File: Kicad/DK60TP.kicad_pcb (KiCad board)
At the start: 2 copper layers, 285 x 113.5 mm, 333 parts, among them J1 USB_mini_micro_B, J2 RGB, J3 CAPS_LOCK, K0 K00, K10 K10, K100 K01, K110 K11, K120 K21, K130 K31, K140 K41, K141 K41, K20 K20, K200 K02, K21 K20, K210 K12, K220 K22, K230 K32, K240 K42, K241 K42, K30 K30, K300 K03, K31 K30, K310 K13, K320 K23, K330 K33, K340 LMB, K341 LMB, K40 K40, K400 K04, K41 K40, K410 K14, K420 K24, K430 K34, K440 MMB, K4C1 K4C, K500 K05, K510 K15, K520 K25, K530 K35, K540 K45, K600 K06, K610 K16, K620 K26, K630 K36, K640 K46, K641 K46, K642 K46, K643 K46, K700 K07, K710 K17, K720 K27, K730 K37, K740 K47, K800 K08, K810 K18, K820 K28, K830 K38, K840 RMB, K841 RMB, K900 K09, K910 K19, K920 K29, K930 K39, K940 K49, M1 MISC, M2 MISC, P1 MOUSE_BOARD, P2 MAIN_BOARD, P3 TRACKPOINT, SW1 RESET, U0 ATMEGA32U4-MU, U1 PAM2804, Y1 Crystal

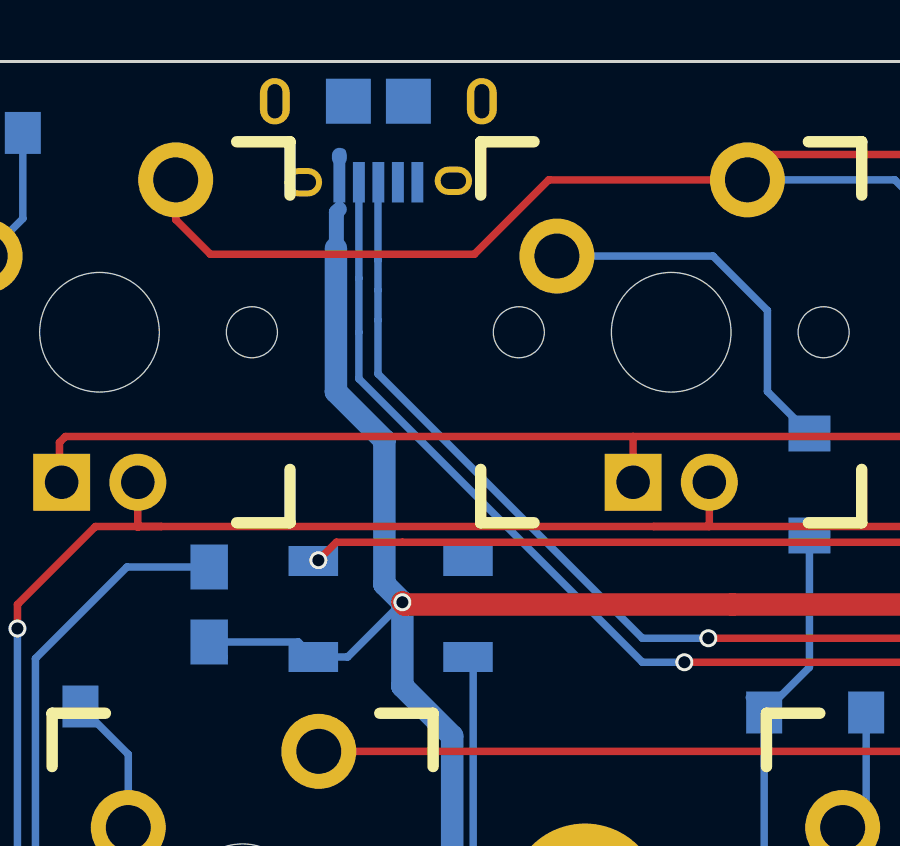
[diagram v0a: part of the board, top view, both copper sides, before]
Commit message: Fixed position of the USB port
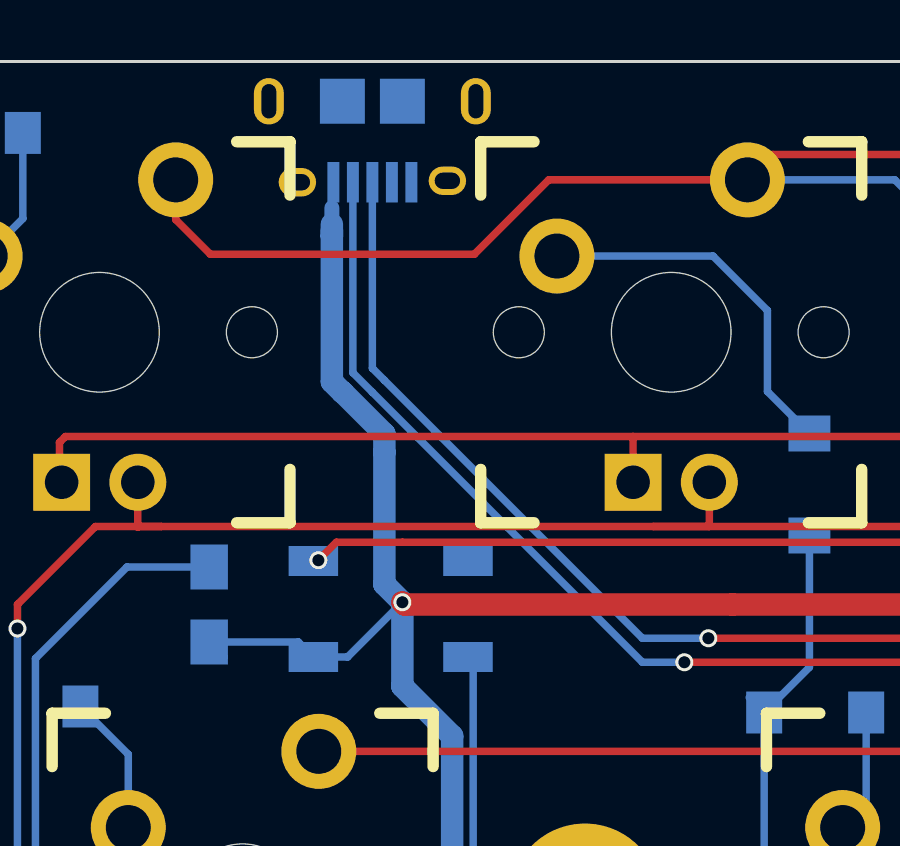
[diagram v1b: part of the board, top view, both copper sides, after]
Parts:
- moved J1 0.20 mm to (82.0, 44.0)
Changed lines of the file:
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@@
     (links 583)
     (no_connects 2)
-    (area 63.881249 39.906249 348.981251 153.506251)
+    (area 44.081251 23.35625 382.58125 192.356251)
     (thickness 1.6)
     (drawings 55)
-    (tracks 2668)
+    (tracks 2666)
     (zones 0)
     (modules 333)
@@
     (38 B.Mask user)
     (39 F.Mask user)
-    (40 Dwgs.User user)
+    (40 Dwgs.User user hide)
     (41 Cmts.User user)
     (42 Eco1.User user)
@@
   )
   (module Footprint:Micro_USB_Hand (layer B.Cu)
-    (at 82.245 43.98125 180)
+    (at 82.045 43.98125 180)
     (fp_text reference J1 (at 0 -2.05 180) (layer B.SilkS)
       (effects (font (size 1 1) (thickness 0.15)) (justify mirror))
@@
   (segment (start 141.931517 126.560413) (end 142.627354 127.25625) (width 0.25) (layer B.Cu) (net 5) (status 10))
   (segment (start 141.909163 126.560413) (end 141.917913 126.560413) (width 0.25) (layer B.Cu) (net 5) (status 30))
+  (segment (start 80.694998 44.831248) (end 80.694998 44.031252) (width 0.25) (layer B.Cu) (net 6) (status 800000))
+  (segment (start 80.694998 44.031252) (end 80.745 43.98125) (width 0.25) (layer B.Cu) (net 6) (status C00000))
+  (segment (start 80.694998 45.38125) (end 80.694998 44.831248) (width 0.5) (layer B.Cu) (net 6))
+  (segment (start 80.694998 45.78125) (end 80.694998 45.38125) (width 0.75) (layer B.Cu) (net 6))
+  (segment (start 81.045 50.98125) (end 81.055048 50.98125) (width 0.75) (layer B.Cu) (net 6))
+  (segment (start 82.445 52.371202) (end 82.445 52.98125) (width 0.75) (layer B.Cu) (net 6))
+  (segment (start 81.055048 50.98125) (end 82.445 52.371202) (width 0.75) (layer B.Cu) (net 6))
+  (segment (start 80.694998 50.631248) (end 80.694998 45.78125) (width 0.75) (layer B.Cu) (net 6))
+  (segment (start 80.694998 45.78125) (end 80.694998 45.58125) (width 0.75) (layer B.Cu) (net 6))
+  (segment (start 81.045 50.98125) (end 80.694998 50.631248) (width 0.75) (layer B.Cu) (net 6))
+  (segment (start 80.745 43.98125) (end 80.745 44.48125) (width 0.25) (layer B.Cu) (net 6) (status C00000))
   (segment (start 80.078 59.80625) (end 81.22 59.80625) (width 0.25) (layer B.Cu) (net 6))
   (segment (start 81.22 59.80625) (end 83.045 57.98125) (width 0.25) (layer B.Cu) (net 6))
@@
   (segment (start 83.12 58.05625) (end 83.045 57.98125) (width 0.75) (layer F.Cu) (net 6))
   (via (at 83.045 57.98125) (size 0.6) (drill 0.4) (layers F.Cu B.Cu) (net 6))
-  (segment (start 82.445 52.58125) (end 80.829375 50.965625) (width 0.75) (layer B.Cu) (net 6))
-  (segment (start 80.845 46.18125) (end 80.829375 46.18125) (width 0.5) (layer B.Cu) (net 6))
-  (segment (start 80.845 44.98125) (end 80.945 44.88125) (width 0.5) (layer B.Cu) (net 6))
-  (segment (start 80.829375 46.18125) (end 80.829375 50.965625) (width 0.75) (layer B.Cu) (net 6))
-  (segment (start 80.945 43.98125) (end 80.945 44.88125) (width 0.25) (layer B.Cu) (net 6))
-  (segment (start 80.845 44.98125) (end 80.845 46.18125) (width 0.5) (layer B.Cu) (net 6))
   (segment (start 83.045 57.98125) (end 82.445 57.38125) (width 0.75) (layer B.Cu) (net 6))
-  (segment (start 82.445 57.38125) (end 82.445 52.58125) (width 0.75) (layer B.Cu) (net 6))
-  (segment (start 80.945 43.18125) (end 80.945 43.08125) (width 0.5) (layer B.Cu) (net 6))
-  (segment (start 80.945 43.98125) (end 80.945 43.18125) (width 0.25) (layer B.Cu) (net 6))
-  (segment (start 80.945 43.08125) (end 81.045 42.98125) (width 0.25) (layer B.Cu) (net 6))
+  (segment (start 82.445 57.38125) (end 82.445 52.98125) (width 0.75) (layer B.Cu) (net 6))
   (segment (start 302.41375 108.85625) (end 302.41375 111.15) (width 0.25) (layer B.Cu) (net 6))
   (segment (start 308.77 117.50625) (end 319.005 117.50625) (width 0.25) (layer B.Cu) (net 6))
@@
   (segment (start 331.705 122.02) (end 331.08375 122.64125) (width 0.25) (layer B.Cu) (net 91) (status 30))
   (segment (start 331.08375 122.64125) (end 333.465 122.64125) (width 0.25) (layer B.Cu) (net 91) (status 30))
+  (segment (start 81.395 43.98125) (end 81.395 50.33125) (width 0.25) (layer B.Cu) (net 92) (status 400000))
+  (segment (start 81.395 50.33125) (end 82.045 50.98125) (width 0.25) (layer B.Cu) (net 92))
   (segment (start 125.445 60.38125) (end 127.81375 62.75) (width 0.25) (layer B.Cu) (net 92))
   (segment (start 127.81375 62.75) (end 127.81375 67.18125) (width 0.25) (layer B.Cu) (net 92))
@@
   (via (at 125.445 60.38125) (size 0.6) (drill 0.4) (layers F.Cu B.Cu) (net 92))
   (segment (start 125.045 59.98125) (end 125.445 60.38125) (width 0.25) (layer F.Cu) (net 92))
-  (segment (start 81.595 48.98125) (end 81.595 50.53125) (width 0.25) (layer B.Cu) (net 92))
-  (segment (start 81.595 50.53125) (end 91.045 59.98125) (width 0.25) (layer B.Cu) (net 92))
+  (segment (start 82.045 50.98125) (end 91.045 59.98125) (width 0.25) (layer B.Cu) (net 92))
   (via (at 92.445 59.98125) (size 0.6) (drill 0.4) (layers F.Cu B.Cu) (net 92))
   (segment (start 91.045 59.98125) (end 92.445 59.98125) (width 0.25) (layer B.Cu) (net 92))
-  (segment (start 81.595 47.18125) (end 81.595 48.98125) (width 0.25) (layer B.Cu) (net 92))
-  (segment (start 81.595 43.98125) (end 81.595 47.18125) (width 0.25) (layer B.Cu) (net 92))
+  (segment (start 82.045 43.98125) (end 82.045 50.18125) (width 0.25) (layer B.Cu) (net 93) (status 400000))
+  (segment (start 82.045 50.18125) (end 82.445 50.58125) (width 0.25) (layer B.Cu) (net 93))
   (segment (start 123.245 59.18125) (end 125.445 59.18125) (width 0.25) (layer F.Cu) (net 93))
   (segment (start 125.445 59.18125) (end 127.045 60.78125) (width 0.25) (layer F.Cu) (net 93))
-  (segment (start 82.23125 48.58125) (end 82.23125 50.3675) (width 0.25) (layer B.Cu) (net 93))
   (segment (start 123.045 59.18125) (end 123.245 59.18125) (width 0.25) (layer F.Cu) (net 93))
   (segment (start 109.445 59.18125) (end 123.045 59.18125) (width 0.25) (layer F.Cu) (net 93))
@@
   (via (at 93.245 59.18125) (size 0.6) (drill 0.4) (layers F.Cu B.Cu) (net 93))
   (segment (start 91.045 59.18125) (end 93.245 59.18125) (width 0.25) (layer B.Cu) (net 93))
-  (segment (start 82.23125 50.3675) (end 91.045 59.18125) (width 0.25) (layer B.Cu) (net 93))
+  (segment (start 82.445 50.58125) (end 91.045 59.18125) (width 0.25) (layer B.Cu) (net 93))
   (segment (start 128.263752 62.000002) (end 128.263752 62.78125) (width 0.25) (layer B.Cu) (net 93))
   (segment (start 127.045 60.78125) (end 128.263752 62.000002) (width 0.25) (layer B.Cu) (net 93))
@@
   (segment (start 128.263752 74.869854) (end 128.263752 62.78125) (width 0.25) (layer B.Cu) (net 93))
   (segment (start 135.109158 81.71526) (end 128.263752 74.869854) (width 0.25) (layer B.Cu) (net 93))
-  (segment (start 82.23125 47.58125) (end 82.23125 48.58125) (width 0.25) (layer B.Cu) (net 93))
-  (segment (start 82.23125 46.58125) (end 82.23125 43.995) (width 0.25) (layer B.Cu) (net 93))
-  (segment (start 82.23125 43.995) (end 82.245 43.98125) (width 0.25) (layer B.Cu) (net 93))
-  (segment (start 82.23125 47.58125) (end 82.23125 46.58125) (width 0.25) (layer B.Cu) (net 93))
   (segment (start 311.445 117.631252) (end 320.194998 117.631252) (width 0.25) (layer F.Cu) (net 94))
   (segment (start 322.578 115.24825) (end 322.578 114.35625) (width 0.25) (layer B.Cu) (net 94))
